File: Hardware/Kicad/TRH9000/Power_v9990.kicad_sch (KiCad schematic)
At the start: 21 parts, among them U1 V9990, U2 KM428C256, U3 KM428C256, U4 74HC138, U6 LMH1980, U7 74HC32

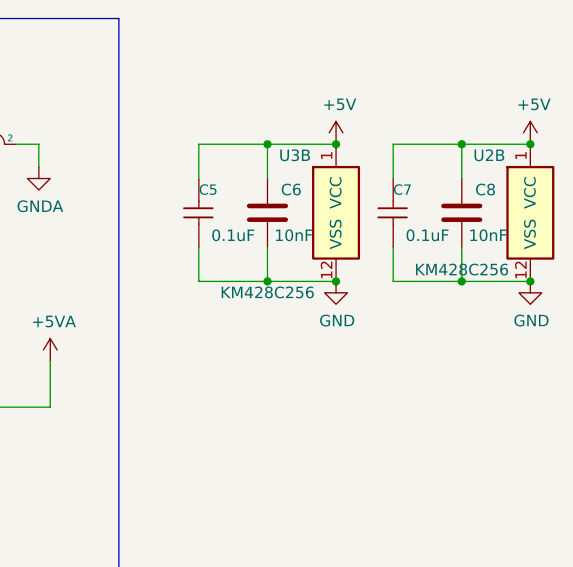
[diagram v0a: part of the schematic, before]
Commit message: Prototype board. Fixes to the main project. Readme updates.
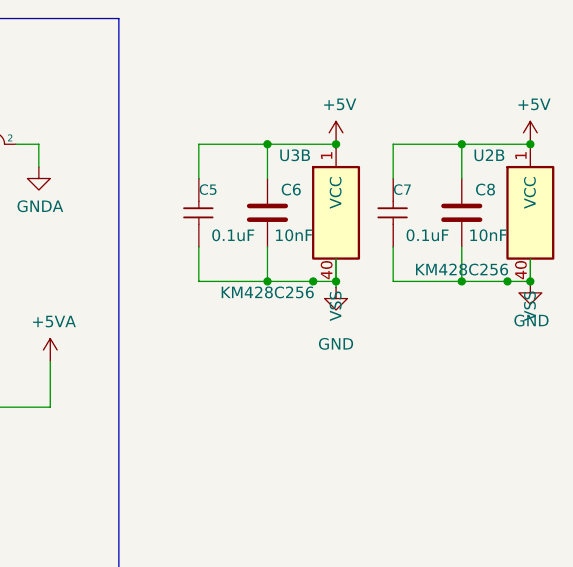
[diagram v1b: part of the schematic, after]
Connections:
- net GND: no longer U2.12 (VSS), U2.21 (VSS), U3.12 (VSS), U3.21 (VSS)
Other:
- moved on the sheet: U2B, U3B
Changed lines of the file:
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@@
   (junction (at 99.06 53.34) (diameter 0) (color 0 0 0 0)
   )
+  (junction (at 222.25 54.61) (diameter 0) (color 0 0 0 0)
+  )
   (junction (at 54.61 53.34) (diameter 0) (color 0 0 0 0)
   )
@@
   (junction (at 157.48 68.58) (diameter 0) (color 0 0 0 0)
   )
+  (junction (at 203.2 54.61) (diameter 0) (color 0 0 0 0)
+  )
+  (junction (at 200.66 54.61) (diameter 0) (color 0 0 0 0)
+  )
   (junction (at 203.2 39.37) (diameter 0) (color 0 0 0 0)
   )
   (junction (at 224.79 39.37) (diameter 0) (color 0 0 0 0)
   )
+  (junction (at 224.79 54.61) (diameter 0) (color 0 0 0 0)
+  )
+  (junction (at 217.17 54.61) (diameter 0) (color 0 0 0 0)
+  )
+  (junction (at 144.78 68.58) (diameter 0) (color 0 0 0 0)
+  )
+  (junction (at 93.98 33.02) (diameter 0) (color 0 0 0 0)
+  )
+  (junction (at 55.88 76.2) (diameter 0) (color 0 0 0 0)
+  )
+  (junction (at 99.06 33.02) (diameter 0) (color 0 0 0 0)
+  )
+  (junction (at 50.8 76.2) (diameter 0) (color 0 0 0 0)
+  )
+  (junction (at 60.96 33.02) (diameter 0) (color 0 0 0 0)
+  )
+  (junction (at 195.58 39.37) (diameter 0) (color 0 0 0 0)
+  )
+  (junction (at 217.17 39.37) (diameter 0) (color 0 0 0 0)
+  )
+  (junction (at 144.78 80.01) (diameter 0) (color 0 0 0 0)
+  )
   (junction (at 195.58 54.61) (diameter 0) (color 0 0 0 0)
   )
-  (junction (at 144.78 68.58) (diameter 0) (color 0 0 0 0)
-  )
-  (junction (at 224.79 54.61) (diameter 0) (color 0 0 0 0)
-  )
-  (junction (at 93.98 33.02) (diameter 0) (color 0 0 0 0)
-  )
-  (junction (at 55.88 76.2) (diameter 0) (color 0 0 0 0)
-  )
-  (junction (at 217.17 54.61) (diameter 0) (color 0 0 0 0)
-  )
-  (junction (at 99.06 33.02) (diameter 0) (color 0 0 0 0)
-  )
-  (junction (at 50.8 76.2) (diameter 0) (color 0 0 0 0)
-  )
-  (junction (at 203.2 54.61) (diameter 0) (color 0 0 0 0)
-  )
-  (junction (at 60.96 33.02) (diameter 0) (color 0 0 0 0)
-  )
-  (junction (at 195.58 39.37) (diameter 0) (color 0 0 0 0)
-  )
-  (junction (at 217.17 39.37) (diameter 0) (color 0 0 0 0)
-  )
-  (junction (at 144.78 80.01) (diameter 0) (color 0 0 0 0)
-  )
   (junction (at 54.61 91.44) (diameter 0) (color 0 0 0 0)
   )
@@
     (stroke (width 0) (type default) (color 0 0 0 0))
   )
-  (wire (pts (xy 217.17 54.61) (xy 224.79 54.61))
-    (stroke (width 0) (type default) (color 0 0 0 0))
-  )
   (polyline (pts (xy 179.07 25.4) (xy 179.07 90.17))
     (stroke (width 0) (type default) (color 0 0 0 0))
@@
     (stroke (width 0) (type default) (color 0 0 0 0))
   )
+  (wire (pts (xy 203.2 52.07) (xy 203.2 54.61))
+    (stroke (width 0) (type default) (color 0 0 0 0))
+  )
   (wire (pts (xy 157.48 80.01) (xy 157.48 78.74))
     (stroke (width 0) (type default) (color 0 0 0 0))
@@
     (stroke (width 0) (type default) (color 0 0 0 0))
   )
+  (wire (pts (xy 203.2 54.61) (xy 203.2 55.245))
+    (stroke (width 0) (type default) (color 0 0 0 0))
+  )
   (wire (pts (xy 52.07 157.48) (xy 52.07 154.94))
     (stroke (width 0) (type default) (color 0 0 0 0))
@@
     (stroke (width 0) (type default) (color 0 0 0 0))
   )
+  (wire (pts (xy 217.17 54.61) (xy 222.25 54.61))
+    (stroke (width 0) (type default) (color 0 0 0 0))
+  )
   (polyline (pts (xy 77.47 25.4) (xy 110.49 25.4))
     (stroke (width 0) (type default) (color 0 0 0 0))
@@
     (stroke (width 0) (type default) (color 0 0 0 0))
   )
+  (wire (pts (xy 224.79 52.07) (xy 224.79 54.61))
+    (stroke (width 0) (type default) (color 0 0 0 0))
+  )
   (wire (pts (xy 93.98 53.34) (xy 99.06 53.34))
     (stroke (width 0) (type default) (color 0 0 0 0))
@@
     (stroke (width 0) (type default) (color 0 0 0 0))
   )
+  (wire (pts (xy 200.66 54.61) (xy 203.2 54.61))
+    (stroke (width 0) (type default) (color 0 0 0 0))
+  )
   (wire (pts (xy 157.48 68.58) (xy 171.45 68.58))
     (stroke (width 0) (type default) (color 0 0 0 0))
@@
     (stroke (width 0) (type default) (color 0 0 0 0))
   )
+  (wire (pts (xy 195.58 54.61) (xy 200.66 54.61))
+    (stroke (width 0) (type default) (color 0 0 0 0))
+  )
   (wire (pts (xy 54.61 50.8) (xy 54.61 53.34))
     (stroke (width 0) (type default) (color 0 0 0 0))
@@
     (stroke (width 0) (type default) (color 0 0 0 0))
   )
+  (wire (pts (xy 222.25 54.61) (xy 224.79 54.61))
+    (stroke (width 0) (type default) (color 0 0 0 0))
+  )
   (wire (pts (xy 105.41 46.99) (xy 105.41 53.34))
     (stroke (width 0) (type default) (color 0 0 0 0))
@@
   )
   (wire (pts (xy 55.88 76.2) (xy 64.77 76.2))
-    (stroke (width 0) (type default) (color 0 0 0 0))
-  )
-  (wire (pts (xy 195.58 54.61) (xy 203.2 54.61))
     (stroke (width 0) (type default) (color 0 0 0 0))
   )
@@
     (pin "2")
   )
-  (symbol (lib_id "TRH9000:KM428C256") (at 203.2 46.99 0) (unit 2)
+  (symbol (lib_name "KM428C256_1") (lib_id "TRH9000:KM428C256") (at 203.2 46.99 0) (unit 2)
     (in_bom yes) (on_board yes)
     (property "Reference" "U3" (id 0) (at 196.85 40.64 0)
@@
     )
     (property "Value" "KM428C256" (id 1) (at 195.58 55.88 0))
-    (property "Footprint" "trh9000:SOJ-40_400mil" (id 2) (at 203.2 57.15 0)
-      (effects (font (size 1.27 1.27)) hide)
-    )
-    (property "Datasheet" "https://pdf1.alldatasheet.com/datasheet-pdf/view/129863/SAMSUNG/KM428C256.html" (id 3) (at 203.2 57.15 0)
+    (property "Footprint" "trh9000:SOJ-40_400mil" (id 2) (at 218.44 83.82 0)
+      (effects (font (size 1.27 1.27)) hide)
+    )
+    (property "Datasheet" "https://pdf1.alldatasheet.com/datasheet-pdf/view/129863/SAMSUNG/KM428C256.html" (id 3) (at 203.2 86.36 0)
       (effects (font (size 1.27 1.27)) hide)
     )
@@
     (pin "10")
     (pin "11")
-    (pin "13")
+    (pin "12")
     (pin "14")
     (pin "15")
@@
     (pin "9")
     (pin "1")
-    (pin "12")
+    (pin "13")
     (pin "20")
     (pin "21")
@@
     )
     (property "Value" "KM428C256" (id 1) (at 217.17 53.34 0))
-    (property "Footprint" "trh9000:SOJ-40_400mil" (id 2) (at 224.79 57.15 0)
-      (effects (font (size 1.27 1.27)) hide)
-    )
-    (property "Datasheet" "https://pdf1.alldatasheet.com/datasheet-pdf/view/129863/SAMSUNG/KM428C256.html" (id 3) (at 224.79 57.15 0)
+    (property "Footprint" "trh9000:SOJ-40_400mil" (id 2) (at 240.03 83.82 0)
+      (effects (font (size 1.27 1.27)) hide)
+    )
+    (property "Datasheet" "https://pdf1.alldatasheet.com/datasheet-pdf/view/129863/SAMSUNG/KM428C256.html" (id 3) (at 224.79 86.36 0)
       (effects (font (size 1.27 1.27)) hide)
     )
@@
     (pin "10")
     (pin "11")
-    (pin "13")
+    (pin "12")
     (pin "14")
     (pin "15")
@@
     (pin "9")
     (pin "1")
-    (pin "12")
+    (pin "13")
     (pin "20")
     (pin "21")
@@
     (pin "1")
   )
-  (symbol (lib_id "power:GND") (at 203.2 54.61 0) (unit 1)
-    (in_bom yes) (on_board yes)
-    (property "Reference" "#PWR0117" (id 0) (at 203.2 60.96 0)
-      (effects (font (size 1.27 1.27)) hide)
-    )
-    (property "Value" "GND" (id 1) (at 203.327 59.0042 0))
-    (property "Footprint" "" (id 2) (at 203.2 54.61 0)
-      (effects (font (size 1.27 1.27)) hide)
-    )
-    (property "Datasheet" "" (id 3) (at 203.2 54.61 0)
-      (effects (font (size 1.27 1.27)) hide)
-    )
+  (symbol (lib_id "power:GND") (at 203.2 55.245 0) (unit 1)
+    (in_bom yes) (on_board yes)
+    (property "Reference" "#PWR0117" (id 0) (at 203.2 61.595 0)
+      (effects (font (size 1.27 1.27)) hide)
+    )
+    (property "Value" "GND" (id 1) (at 203.2 61.595 0))
+    (property "Footprint" "" (id 2) (at 203.2 55.245 0)
+      (effects (font (size 1.27 1.27)) hide)
+    )
+    (property "Datasheet" "" (id 3) (at 203.2 55.245 0)
+      (effects (font (size 1.27 1.27)) hide)
+    )
